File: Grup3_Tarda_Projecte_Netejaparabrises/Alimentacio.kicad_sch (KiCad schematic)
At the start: 14 parts, among them IC1 L78S05CV, J1 Screw_Terminal_01x02

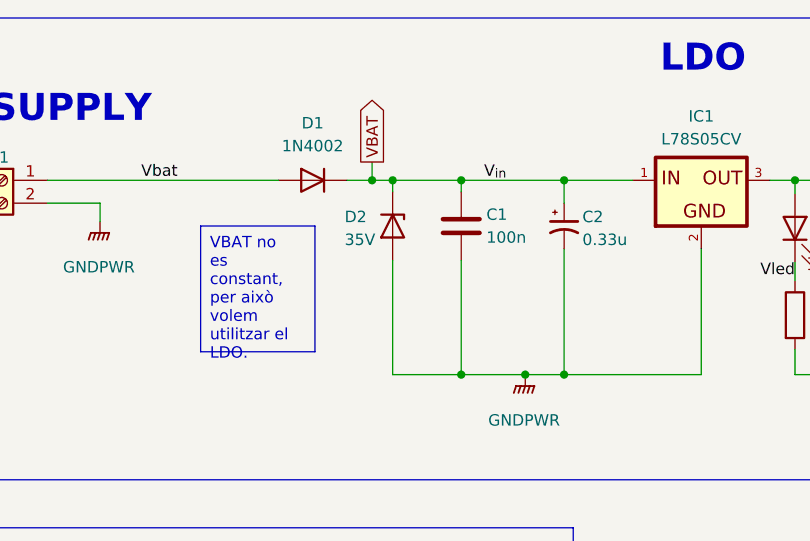
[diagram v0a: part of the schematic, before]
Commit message: routing v1 sense acabar
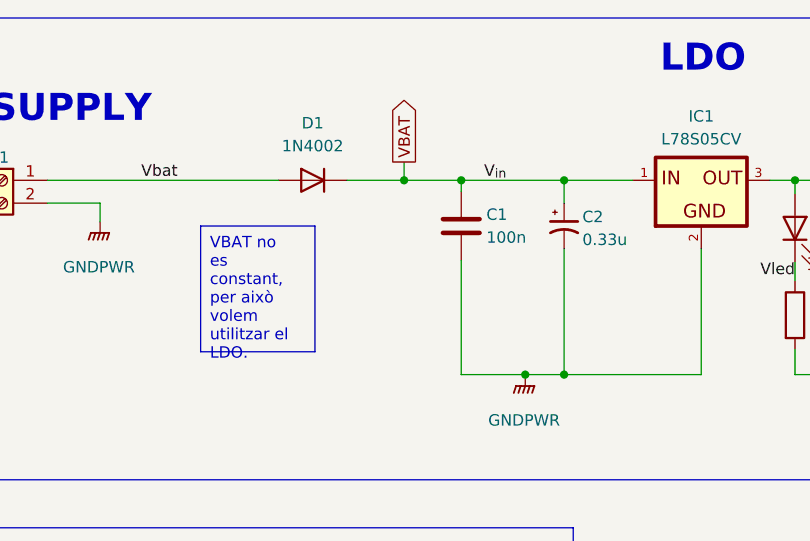
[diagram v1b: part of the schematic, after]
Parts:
- removed D2: 35V, Diode_THT:D_5W_P5.08mm_Vertical_AnodeUp, symbol Device:D_Zener
- C1, C5: footprint Capacitor_SMD:C_0805_2012Metric -> Capacitor_THT:C_Disc_D3.0mm_W1.6mm_P2.50mm
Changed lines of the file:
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@@
   (junction (at 132.334 62.992) (diameter 0) (color 0 0 0 0)
   )
-  (junction (at 113.284 62.992) (diameter 0) (color 0 0 0 0)
-  )
-  (junction (at 120.904 84.582) (diameter 0) (color 0 0 0 0)
-  )
   (junction (at 132.334 84.582) (diameter 0) (color 0 0 0 0)
   )
@@
   (junction (at 128.016 84.582) (diameter 0) (color 0 0 0 0)
   )
-  (junction (at 110.998 62.992) (diameter 0) (color 0 0 0 0)
-  )
   (junction (at 77.47 132.08) (diameter 0) (color 0 0 0 0)
   )
@@
   (junction (at 77.47 124.46) (diameter 0) (color 0 0 0 0)
   )
+  (junction (at 114.554 62.992) (diameter 0) (color 0 0 0 0)
+  )
   (wire (pts (xy 120.904 84.582) (xy 128.016 84.582))
     (stroke (width 0) (type default))
@@
     (stroke (width 0) (type default))
   )
-  (wire (pts (xy 113.284 71.882) (xy 113.284 84.582))
+  (wire (pts (xy 114.554 62.992) (xy 120.904 62.992))
     (stroke (width 0) (type default))
   )
@@
     (stroke (width 0) (type default))
   )
-  (wire (pts (xy 113.284 62.992) (xy 120.904 62.992))
-    (stroke (width 0) (type default))
-  )
   (wire (pts (xy 120.904 62.992) (xy 132.334 62.992))
     (stroke (width 0) (type default))
@@
     (stroke (width 0) (type default))
   )
-  (wire (pts (xy 113.284 84.582) (xy 120.904 84.582))
-    (stroke (width 0) (type default))
-  )
   (wire (pts (xy 167.894 62.992) (xy 178.054 62.992))
     (stroke (width 0) (type default))
@@
     (stroke (width 0) (type default))
   )
-  (wire (pts (xy 108.204 62.992) (xy 110.998 62.992))
+  (wire (pts (xy 108.204 62.992) (xy 114.554 62.992))
     (stroke (width 0) (type default))
   )
@@
     (stroke (width 0) (type default))
   )
-  (wire (pts (xy 113.284 62.992) (xy 113.284 64.262))
-    (stroke (width 0) (type default))
-  )
-  (wire (pts (xy 110.998 60.96) (xy 110.998 62.992))
+  (wire (pts (xy 114.554 60.96) (xy 114.554 62.992))
     (stroke (width 0) (type default))
   )
@@
   )
   (wire (pts (xy 111.76 134.62) (xy 111.76 133.35))
-    (stroke (width 0) (type default))
-  )
-  (wire (pts (xy 110.998 62.992) (xy 113.284 62.992))
     (stroke (width 0) (type default))
   )
@@
     )
   )
-  (global_label "VBAT" (shape output) (at 110.998 60.96 90) (fields_autoplaced)
+  (global_label "VBAT" (shape output) (at 114.554 60.96 90) (fields_autoplaced)
     (effects (font (size 1.27 1.27)) (justify left))
-    (property "Intersheetrefs" "${INTERSHEET_REFS}" (at 110.998 53.6394 90)
+    (property "Intersheetrefs" "${INTERSHEET_REFS}" (at 114.554 53.6394 90)
       (effects (font (size 1.27 1.27)) (justify left) hide)
     )
@@
       (effects (font (size 1.27 1.27)) (justify left))
     )
-    (property "Footprint" "Capacitor_SMD:C_0805_2012Metric" (at 121.8692 71.882 0)
+    (property "Footprint" "Capacitor_THT:C_Disc_D3.0mm_W1.6mm_P2.50mm" (at 121.8692 71.882 0)
       (effects (font (size 1.27 1.27)) hide)
     )
@@
       (effects (font (size 1.27 1.27)) (justify left))
     )
-    (property "Footprint" "Capacitor_SMD:C_0805_2012Metric" (at 179.0192 72.136 0)
+    (property "Footprint" "Capacitor_THT:C_Disc_D3.0mm_W1.6mm_P2.50mm" (at 179.0192 72.136 0)
       (effects (font (size 1.27 1.27)) hide)
     )
@@
         )
       )
-    )
-  )
-  (symbol (lib_id "Device:D_Zener") (at 113.284 68.072 270) (unit 1)
-    (in_bom yes) (on_board yes) (dnp no)
-    (property "Reference" "D2" (at 107.95 67.0559 90)
-      (effects (font (size 1.27 1.27)) (justify left))
-    )
-    (property "Value" "35V" (at 107.95 69.596 90)
-      (effects (font (size 1.27 1.27)) (justify left))
-    )
-    (property "Footprint" "Diode_THT:D_5W_P5.08mm_Vertical_AnodeUp" (at 113.284 68.072 0)
-      (effects (font (size 1.27 1.27)) hide)
-    )
-    (property "Datasheet" "~" (at 113.284 68.072 0)
-      (effects (font (size 1.27 1.27)) hide)
-    )
-    (pin "1")
-    (pin "2")
-    (instances
-      (project ""
-        (path "/471896f9-a17e-46cb-bb6a-e6efc81f054f"
-          (reference "D2") (unit 1)
-        )
-      )
-      (project "Grup3_Tarda_Projecte_Netejaparabrises"
-        (path "/7ae78f34-680b-4fd9-8391-ce3e1c73c4b5"
-          (reference "D2") (unit 1)
-        )
-        (path "/7ae78f34-680b-4fd9-8391-ce3e1c73c4b5/de573664-441d-44bf-8893-2d2e822d4a99"
-          (reference "D2") (unit 1)
-        )
-      )
-      (project "AidarIglesias_DavidMiravent_P3"
-        (path "/f9f603a9-b774-48a7-94d1-4c8d3d65a3f8"
-          (reference "D2") (unit 1)
-        )
-      )
